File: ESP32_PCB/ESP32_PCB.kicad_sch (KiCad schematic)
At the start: 22 parts, among them J1 USB_C_Receptacle, J2 ESC1, J3 ESC2, U1 ESP32-S3-MINI-1, U2 H3LIS331DL, U3 AP2112K-3.3

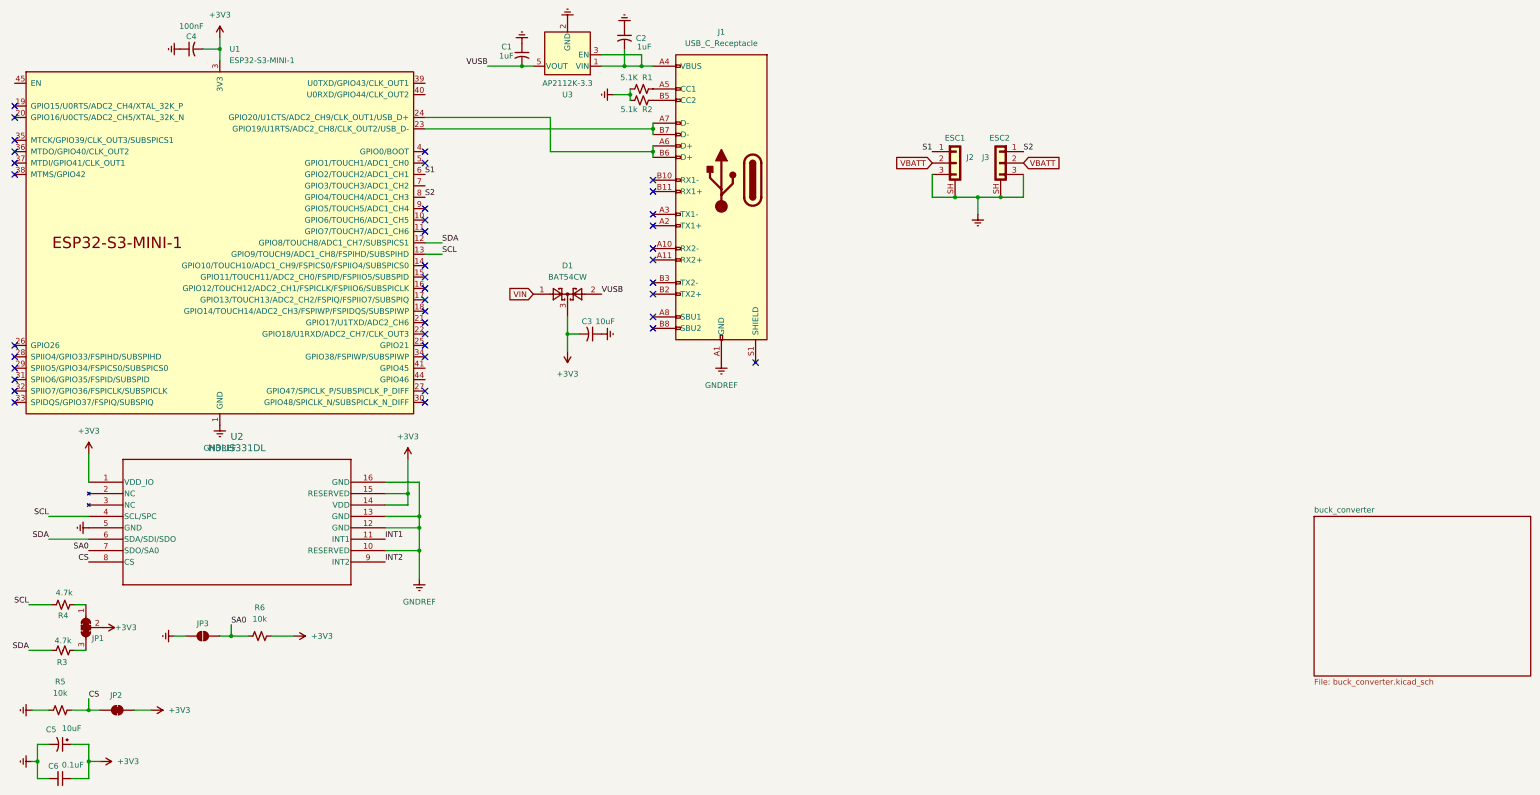
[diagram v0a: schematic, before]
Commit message: start pcb
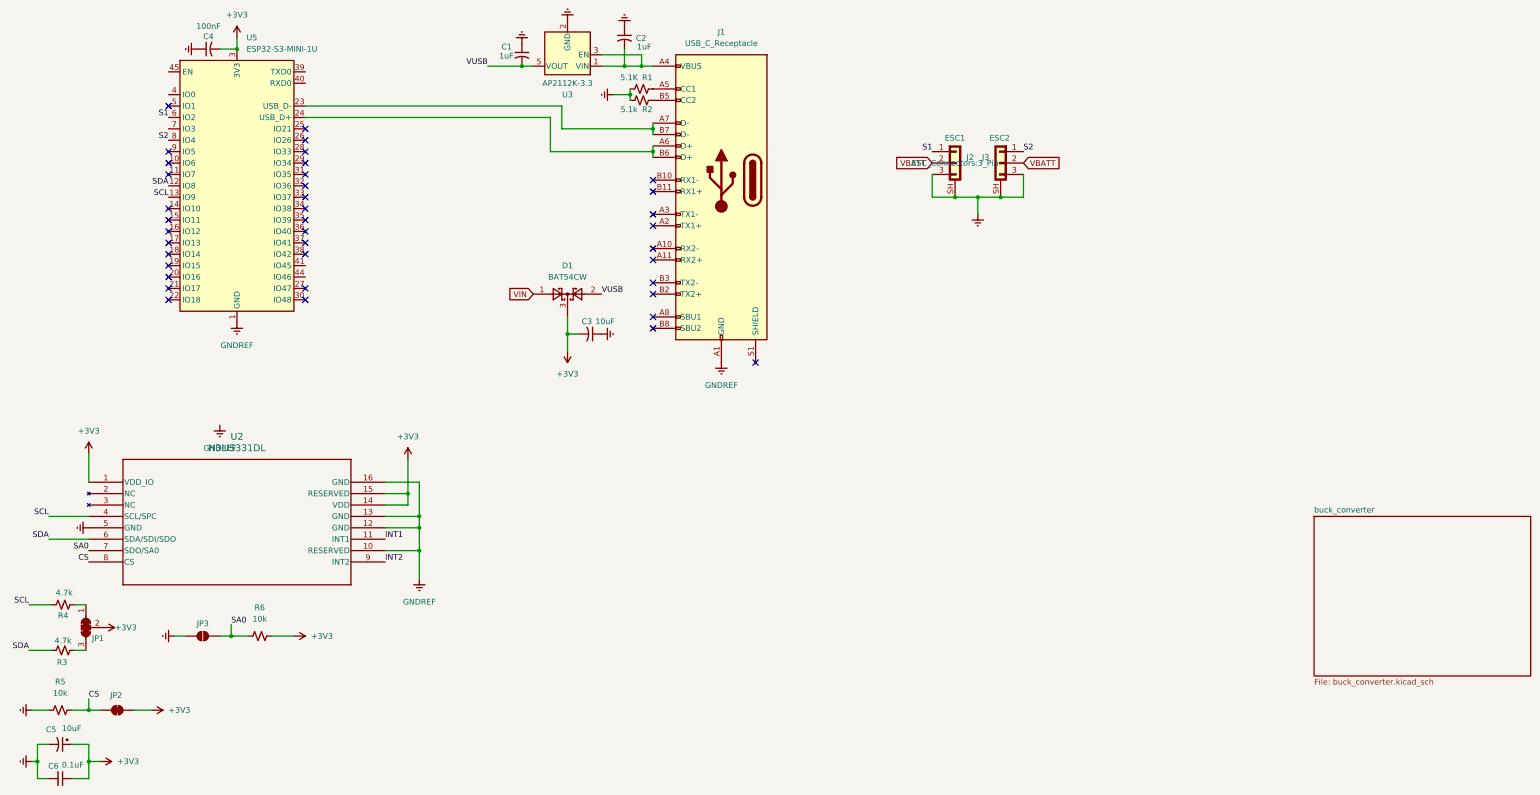
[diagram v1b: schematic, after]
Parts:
- removed U1: ESP32-S3-MINI-1, PCM_Espressif:ESP32-S3-MINI-1, symbol PCM_Espressif:ESP32-S3-MINI-1
- added U5: ESP32-S3-MINI-1U, RF_Module:ESP32-S2-MINI-1U, symbol RF_Module:ESP32-S3-MINI-1U
- C5: footprint Capacitor_SMD:CP_Elec_3x5.3 -> Capacitor_Tantalum_SMD:CP_EIA-1608-08_AVX-J
- J2, J3: footprint (none) -> ESC_Connectors:3_Pin
- U2: footprint TFLGA16_3X3X1_STM -> accelerometer:TFLGA16_3X3X1_STM
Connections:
- net +3V3: now also U5.3 (3V3)
- net GNDREF: now also U5.1 (GND), U5.2 (GND), U5.42 (GND), U5.43 (GND), U5.46 (GND), U5.47 (GND), U5.48 (GND), U5.49 (GND), U5.50 (GND), U5.51 (GND), U5.52 (GND), U5.53 (GND), U5.54 (GND), U5.55 (GND), U5.56 (GND), U5.57 (GND), U5.58 (GND), U5.59 (GND), U5.60 (GND), U5.61 (GND), U5.62 (GND), U5.63 (GND), U5.64 (GND), U5.65 (GND)
- net S1: now also U5.6 (IO2)
- net S2: now also U5.8 (IO4)
- net SCL: now also U5.13 (IO9)
- net SDA: now also U5.12 (IO8)
- net at J1.A7 (D-), J1.B7 (D-): now also U5.23 (USB_D-)
- net at J1.A6 (D+), J1.B6 (D+): now also U5.24 (USB_D+)
- no-connect marks 39 -> 38
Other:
- moved on the sheet: C4
